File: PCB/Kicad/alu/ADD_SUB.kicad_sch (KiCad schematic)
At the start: 18 parts, among them U17 7486, U18 7486, U19 7486, U20 74283, U21 74283, U22 7486, U23 7486, U24 74283, U25 74283

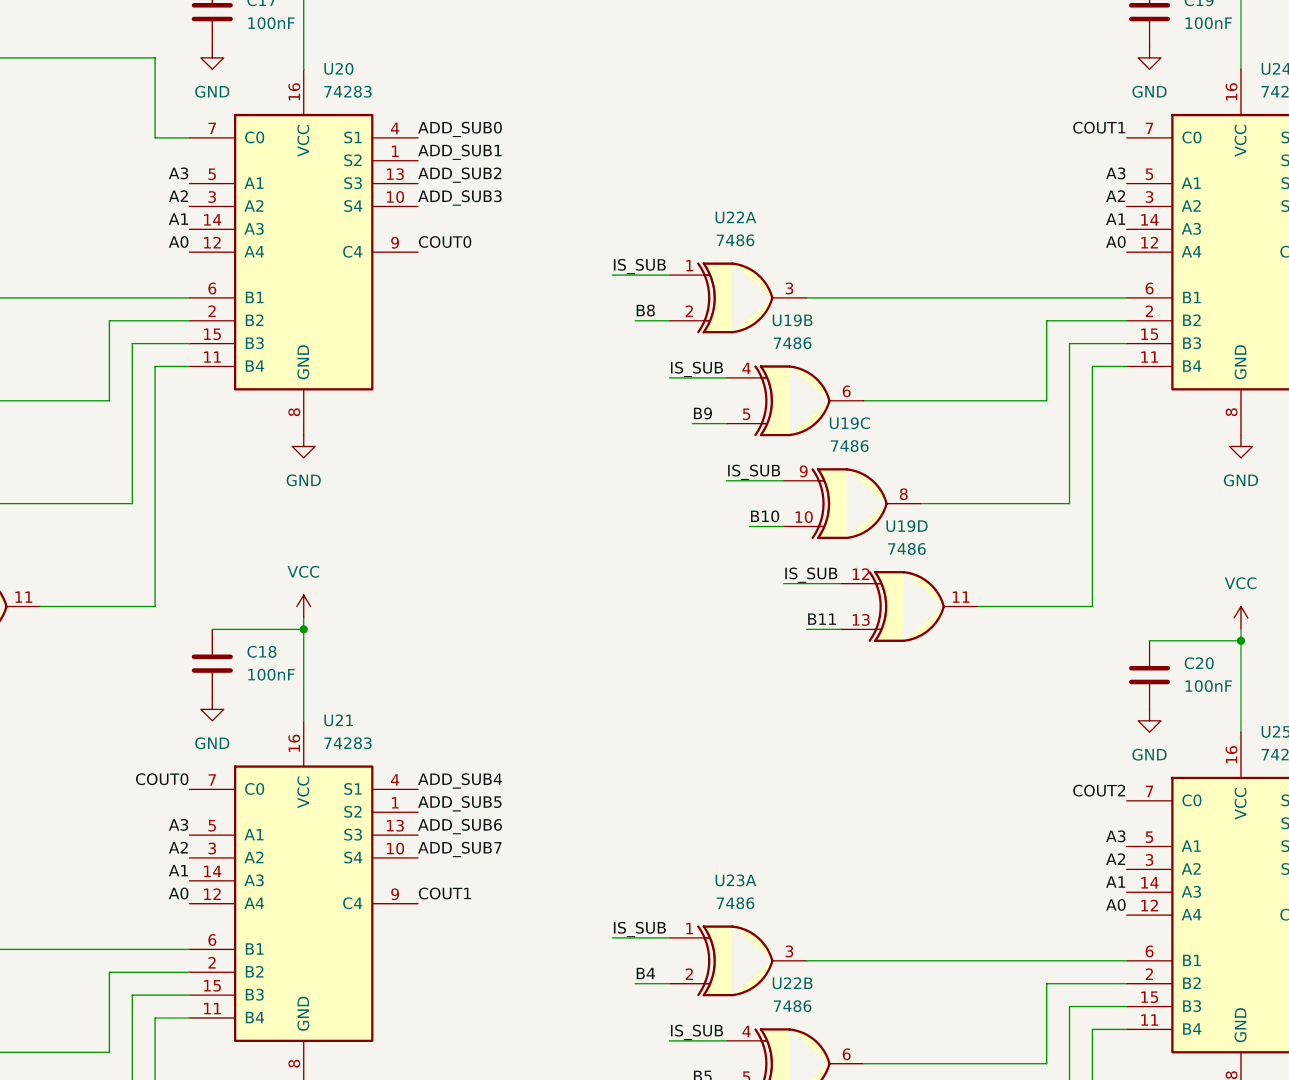
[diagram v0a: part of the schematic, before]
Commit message: PCB
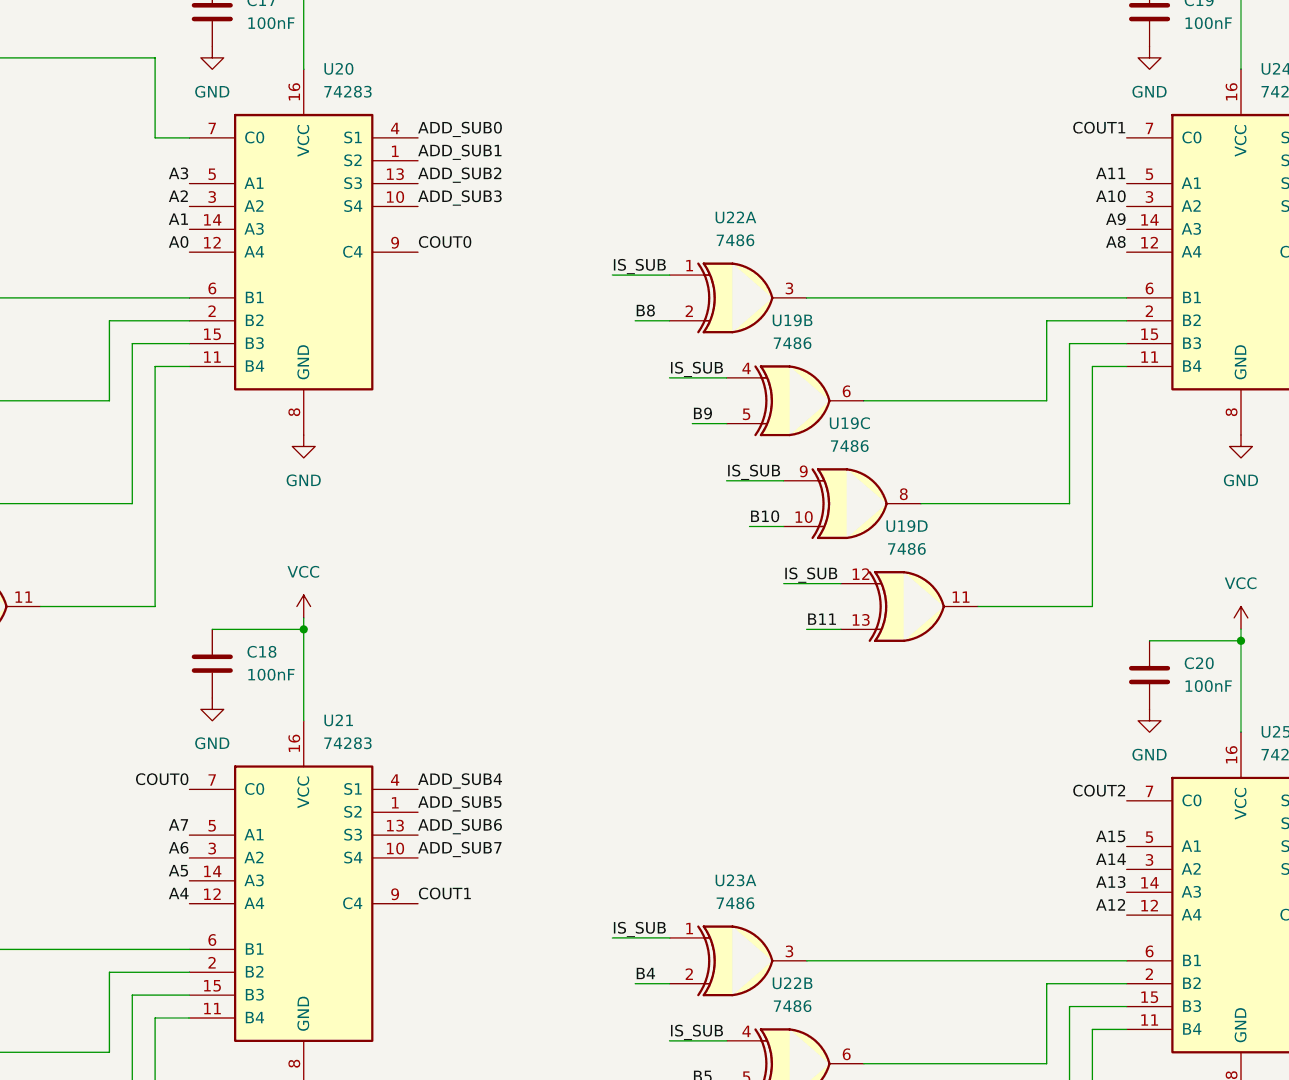
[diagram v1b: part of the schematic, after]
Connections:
- net A0: no longer U21.12 (A4), U24.12 (A4), U25.12 (A4)
- net A1: no longer U21.14 (A3), U24.14 (A3), U25.14 (A3)
- net A2: no longer U21.3 (A2), U24.3 (A2), U25.3 (A2)
- net A3: no longer U21.5 (A1), U24.5 (A1), U25.5 (A1)
- new net A10: U24.3 (A2)
- new net A11: U24.5 (A1)
- new net A12: U25.12 (A4)
- new net A13: U25.14 (A3)
- new net A14: U25.3 (A2)
- new net A15: U25.5 (A1)
- new net A4: U21.12 (A4)
- new net A5: U21.14 (A3)
- new net A6: U21.3 (A2)
- new net A7: U21.5 (A1)
- new net A8: U24.12 (A4)
- new net A9: U24.14 (A3)
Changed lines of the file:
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@@
 		)
 	)
-	(label "A2"
+	(label "A6"
 		(at 77.47 119.38 180)
 		(effects
@@
 		)
 	)
-	(label "A0"
+	(label "A12"
 		(at 181.61 125.73 180)
 		(effects
@@
 		)
 	)
-	(label "A1"
+	(label "A9"
 		(at 181.61 49.53 180)
 		(effects
@@
 		)
 	)
-	(label "A3"
+	(label "A15"
 		(at 181.61 118.11 180)
 		(effects
@@
 		)
 	)
-	(label "A3"
+	(label "A11"
 		(at 181.61 44.45 180)
 		(effects
@@
 		)
 	)
-	(label "A2"
+	(label "A10"
 		(at 181.61 46.99 180)
 		(effects
@@
 		)
 	)
-	(label "A1"
+	(label "A5"
 		(at 77.47 121.92 180)
 		(effects
@@
 		)
 	)
-	(label "A0"
+	(label "A4"
 		(at 77.47 124.46 180)
 		(effects
@@
 		)
 	)
-	(label "A3"
+	(label "A7"
 		(at 77.47 116.84 180)
 		(effects
@@
 		)
 	)
-	(label "A2"
+	(label "A14"
 		(at 181.61 120.65 180)
 		(effects
@@
 		)
 	)
-	(label "A0"
+	(label "A8"
 		(at 181.61 52.07 180)
 		(effects
@@
 		)
 	)
-	(label "A1"
+	(label "A13"
 		(at 181.61 123.19 180)
 		(effects

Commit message: Stuff and layout
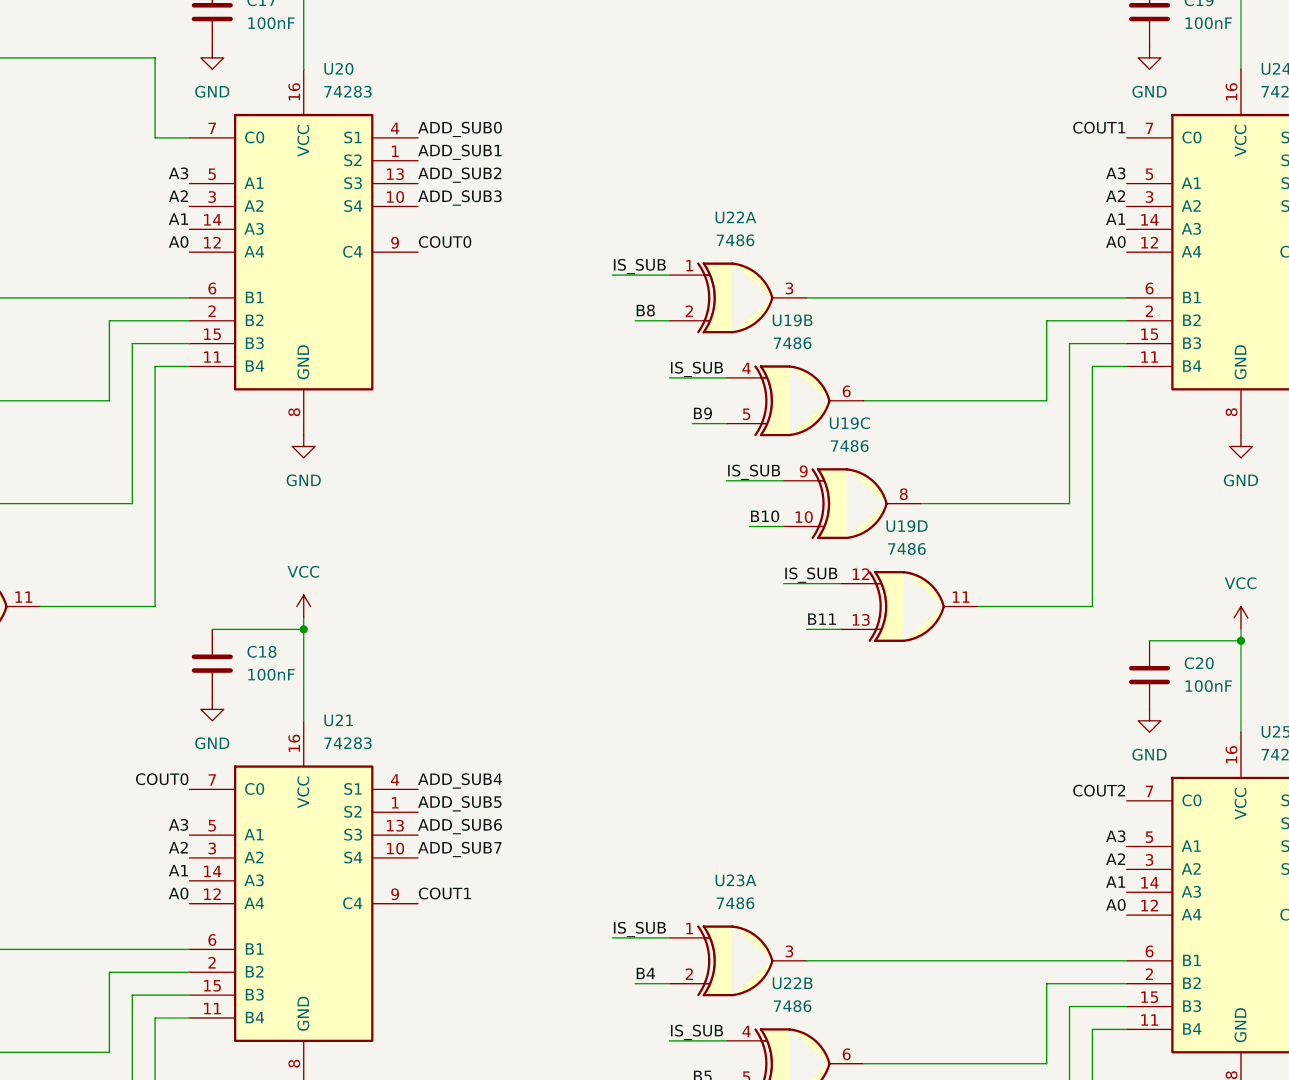
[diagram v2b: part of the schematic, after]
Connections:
- net A10 is gone; now on net A2: U24.3 (A2)
- net A11 is gone; now on net A3: U24.5 (A1)
- net A12 is gone; now on net A0: U25.12 (A4)
- net A13 is gone; now on net A1: U25.14 (A3)
- net A14 is gone; now on net A2: U25.3 (A2)
- net A15 is gone; now on net A3: U25.5 (A1)
- net A4 is gone; now on net A0: U21.12 (A4)
- net A5 is gone; now on net A1: U21.14 (A3)
- net A6 is gone; now on net A2: U21.3 (A2)
- net A7 is gone; now on net A3: U21.5 (A1)
- net A8 is gone; now on net A0: U24.12 (A4)
- net A9 is gone; now on net A1: U24.14 (A3)
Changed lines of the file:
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@@
 		)
 	)
-	(label "A6"
+	(label "A2"
 		(at 77.47 119.38 180)
 		(effects
@@
 		)
 	)
-	(label "A12"
+	(label "A0"
 		(at 181.61 125.73 180)
 		(effects
@@
 		)
 	)
-	(label "A9"
+	(label "A1"
 		(at 181.61 49.53 180)
 		(effects
@@
 		)
 	)
-	(label "A15"
+	(label "A3"
 		(at 181.61 118.11 180)
 		(effects
@@
 		)
 	)
-	(label "A11"
+	(label "A3"
 		(at 181.61 44.45 180)
 		(effects
@@
 		)
 	)
-	(label "A10"
+	(label "A2"
 		(at 181.61 46.99 180)
 		(effects
@@
 		)
 	)
-	(label "A5"
+	(label "A1"
 		(at 77.47 121.92 180)
 		(effects
@@
 		)
 	)
-	(label "A4"
+	(label "A0"
 		(at 77.47 124.46 180)
 		(effects
@@
 		)
 	)
-	(label "A7"
+	(label "A3"
 		(at 77.47 116.84 180)
 		(effects
@@
 		)
 	)
-	(label "A14"
+	(label "A2"
 		(at 181.61 120.65 180)
 		(effects
@@
 		)
 	)
-	(label "A8"
+	(label "A0"
 		(at 181.61 52.07 180)
 		(effects
@@
 		)
 	)
-	(label "A13"
+	(label "A1"
 		(at 181.61 123.19 180)
 		(effects
